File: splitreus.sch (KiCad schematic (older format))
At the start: 93 parts, among them SW0 SW_PUSH, SW1 SW_PUSH, SW10 SW_PUSH, SW11 SW_PUSH, SW12 SW_PUSH, SW13 SW_PUSH, SW14 SW_PUSH, SW15 SW_PUSH, SW16 SW_PUSH, SW17 SW_PUSH, SW18 SW_PUSH, SW19 SW_PUSH, SW2 SW_PUSH, SW20 SW_PUSH, SW21 SW_PUSH, SW22 SW_PUSH, SW23 SW_PUSH, SW24 SW_PUSH, SW25 SW_PUSH, SW26 SW_PUSH, SW27 SW_PUSH, SW28 SW_PUSH, SW29 SW_PUSH, SW3 SW_PUSH, SW30 SW_PUSH, SW4 SW_PUSH, SW5 SW_PUSH, SW6 SW_PUSH, SW7 SW_PUSH, SW8 SW_PUSH, SW9 SW_PUSH, U1 nice_nano, U10 HOLE, U11 HOLE, U12 HOLE, U13 HOLE, U14 HOLE, U15 HOLE, U16 HOLE, U17 HOLE, U18 HOLE, U19 HOLE, U2 HOLE, U20 HOLE, U21 HOLE, U22 HOLE, U23 HOLE, U24 HOLE, U25 HOLE, U26 HOLE, U27 HOLE, U28 HOLE, U29 HOLE, U3 HOLE, U4 HOLE, U5 HOLE, U6 HOLE, U7 HOLE, U8 HOLE, U9 HOLE

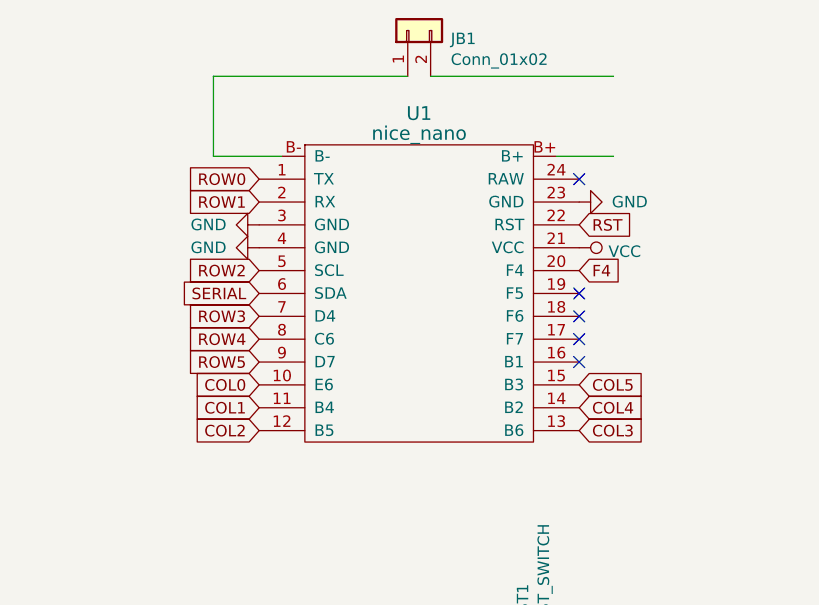
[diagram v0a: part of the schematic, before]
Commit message: semi done
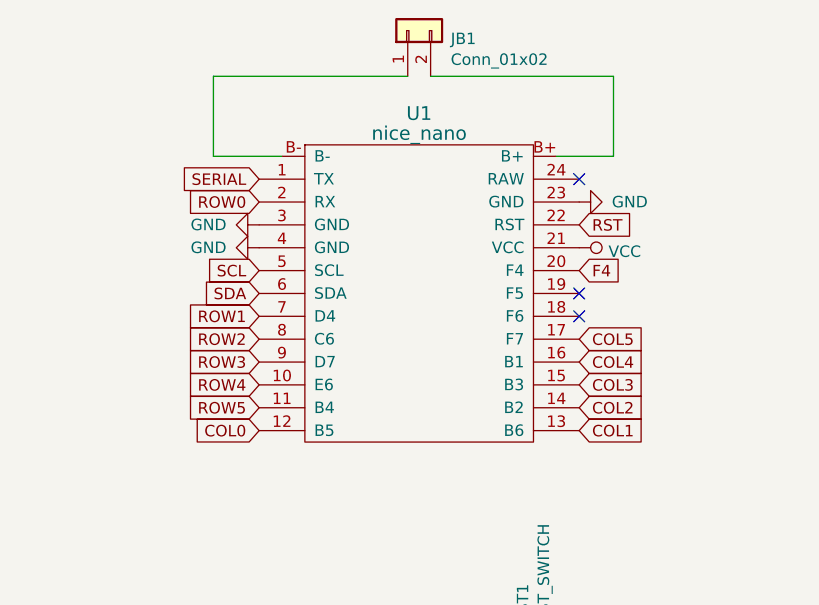
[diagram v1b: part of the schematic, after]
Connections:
- net COL0: now also U1.12 (B5); no longer U1.10 (E6)
- net COL1: now also U1.13 (B6); no longer U1.11 (B4)
- net COL2: now also U1.14 (B2); no longer U1.12 (B5)
- net COL3: now also U1.15 (B3); no longer U1.13 (B6)
- net COL4: now also U1.16 (B1); no longer U1.14 (B2)
- net COL5: now also U1.17 (F7); no longer U1.15 (B3)
- net ROW0: now also U1.2 (RX); no longer U1.1 (TX)
- net ROW1: now also U1.7 (D4); no longer U1.2 (RX)
- net ROW2: now also U1.8 (C6); no longer U1.5 (SCL)
- net ROW3: now also U1.9 (D7); no longer U1.7 (D4)
- net ROW4: now also U1.10 (E6); no longer U1.8 (C6)
- net ROW5: now also U1.11 (B4); no longer U1.9 (D7)
- net SERIAL: now also U1.1 (TX); no longer U1.6 (SDA)
- net at U1.B+: now also JB1.2 (Pin_2)
- new net SCL: U1.5 (SCL)
- new net SDA: U1.6 (SDA)
- no-connect marks 5 -> 3
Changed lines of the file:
@@
 Text GLabel 7400 5700 1    50   Input ~ 0
 ROW5
-Text GLabel 9200 1500 0    50   Input ~ 0
+Text GLabel 9200 1600 0    50   Input ~ 0
 ROW0
-Text GLabel 9200 1600 0    50   Input ~ 0
+Text GLabel 9200 2100 0    50   Input ~ 0
 ROW1
-Text GLabel 9200 1900 0    50   Input ~ 0
+Text GLabel 9200 2200 0    50   Input ~ 0
 ROW2
-Text GLabel 9200 2100 0    50   Input ~ 0
+Text GLabel 9200 2300 0    50   Input ~ 0
 ROW3
-Text GLabel 9200 2200 0    50   Input ~ 0
+Text GLabel 9200 2400 0    50   Input ~ 0
 ROW4
-Text GLabel 9200 2300 0    50   Input ~ 0
+Text GLabel 9200 2500 0    50   Input ~ 0
 ROW5
-Text GLabel 9200 2400 0    50   Input ~ 0
+Text GLabel 9200 2600 0    50   Input ~ 0
 COL0
-Text GLabel 9200 2500 0    50   Input ~ 0
+Text GLabel 10600 2600 2    50   Input ~ 0
 COL1
-Text GLabel 9200 2600 0    50   Input ~ 0
+Text GLabel 10600 2500 2    50   Input ~ 0
 COL2
 Text GLabel 1650 5100 3    50   Input ~ 0
@@
 Text GLabel 7550 6000 3    50   Input ~ 0
 COL5
-Text GLabel 10600 2500 2    50   Input ~ 0
+Text GLabel 10600 2300 2    50   Input ~ 0
 COL4
+Text GLabel 10600 2200 2    50   Input ~ 0
+COL5
+Text GLabel 9200 1500 0    50   Input ~ 0
+SERIAL
 Text GLabel 10600 2400 2    50   Input ~ 0
-COL5
-Text GLabel 9200 2000 0    50   Input ~ 0
-SERIAL
-Text GLabel 10600 2600 2    50   Input ~ 0
 COL3
 Wire Wire Line
@@
 $EndComp
 NoConn ~ 10600 2000
-NoConn ~ 10600 2100
-NoConn ~ 10600 2200
-NoConn ~ 10600 2300
 NoConn ~ 10600 1500
 $Comp
@@
 F 3 "" H 13550 7850 60  0000 C CNN
 	1    13550 7850
-	1    0    0    -1
-$EndComp
-$Comp
-L promicro:nice_nano U1
-U 1 1 5E46BADA
-P 9900 2250
-F 0 "U1" H 9900 3287 60  0000 C CNN
-F 1 "nice_nano" H 9900 3200 60  0000 C CNN
-F 2 "Custom Footies:nice_nano" H 10000 1200 60  0001 C CNN
-F 3 "" H 10000 1200 60  0000 C CNN
-	1    9900 2250
 	1    0    0    -1
 $EndComp
@@
 Wire Wire Line
 	10750 1400 10500 1400
+Wire Wire Line
+	10750 1050 10750 1400
+$Comp
+L promicro:nice_nano U1
+U 1 1 5E46BADA
+P 9900 2250
+F 0 "U1" H 9900 3287 60  0000 C CNN
+F 1 "nice_nano" H 9900 3200 60  0000 C CNN
+F 2 "Custom Footies:nice_nano" H 10000 1200 60  0001 C CNN
+F 3 "" H 10000 1200 60  0000 C CNN
+	1    9900 2250
+	1    0    0    -1
+$EndComp
+NoConn ~ 10600 2100
+Text GLabel 9200 1900 0    50   Input ~ 0
+SCL
+Text GLabel 9200 2000 0    50   Input ~ 0
+SDA
 $EndSCHEMATC
